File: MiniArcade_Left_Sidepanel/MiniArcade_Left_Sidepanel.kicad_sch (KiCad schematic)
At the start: 3 parts, among them J3 USB_C_PWR_Connector

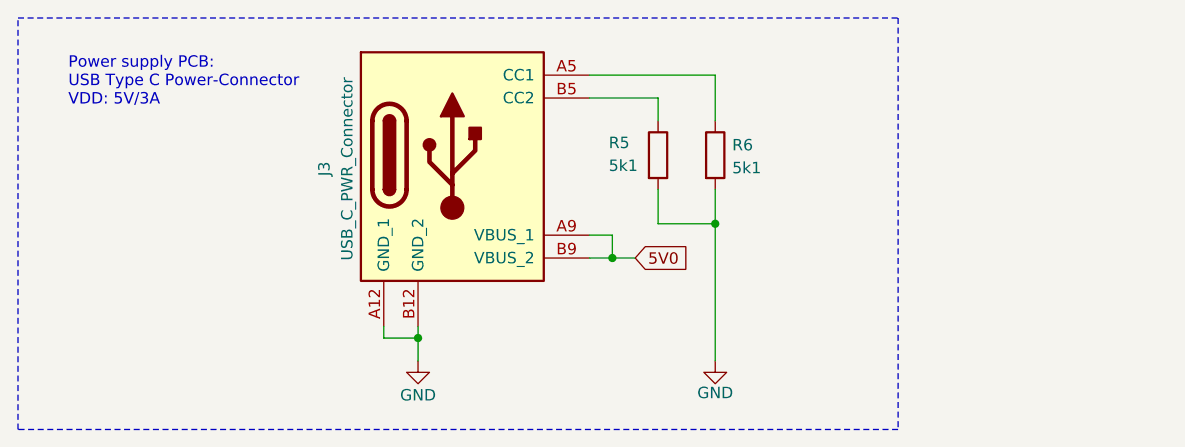
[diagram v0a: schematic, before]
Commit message: 11 11 2025
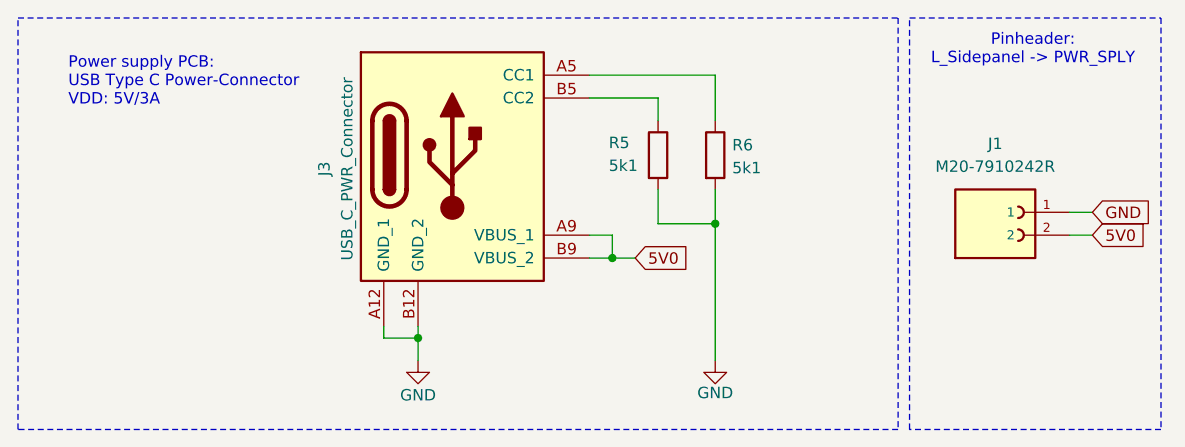
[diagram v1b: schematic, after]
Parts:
- added J1: M20-7910242R, MiniArcadeLeftSidepanel:HARWIN_M20-7910242R, symbol MiniArcadeLeftSidepanel:M20-7910242R
- J3: footprint MiniArcadePWRSupply:USB4125GFA -> MiniArcadeLeftSidepanel:USB4125GFA
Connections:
- net 5V0: now also J1.2
- net GND: now also J1.1
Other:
- note added: "Pinheader: L_Sidepanel -> PWR_SPLY"
